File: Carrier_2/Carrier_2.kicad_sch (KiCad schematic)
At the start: 9 parts, among them J1 HV, J2 3-5V, J3 Out 1, J4 Out 2, U1 LGAD_2_pad

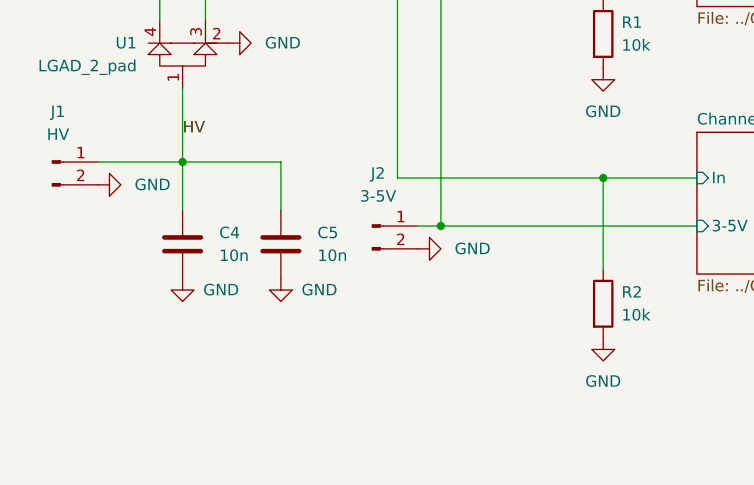
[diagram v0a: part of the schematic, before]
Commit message: Several updates
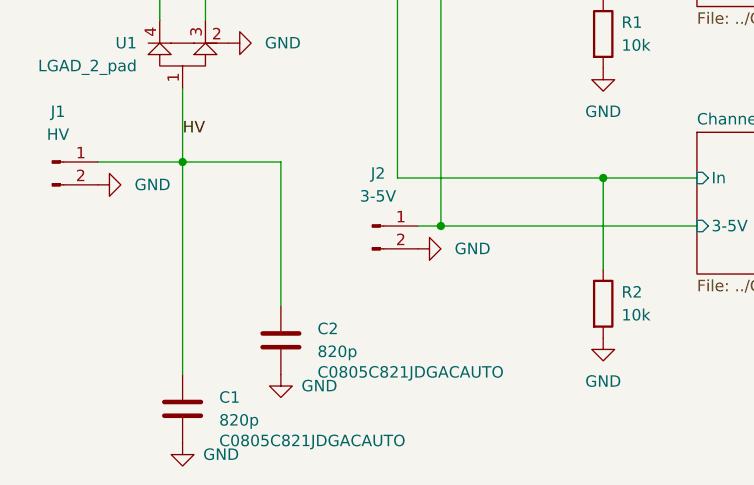
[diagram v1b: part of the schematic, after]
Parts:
- removed C4, C5: 10n, Capacitor_SMD:C_0805_2012Metric, symbol Device:C
- added C1, C2: 820p, Capacitor_SMD:C_0805_2012Metric, symbol Device:C
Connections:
- net GND: now also C1.2, C2.2
- net HV: now also C1.1, C2.1
